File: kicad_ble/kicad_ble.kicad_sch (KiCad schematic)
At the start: 94 parts, among them J2 78171-0002, J3 TC2030_SWD, SW1 RST, SW2 RotaryEncoder_Switch, U1 MAX17048, U2 BQ24075, U3 SRV05-4, U4 nRF52840_E73-2G4M08S1C, U5 74LVC1G11, Y1 32.768 KHz

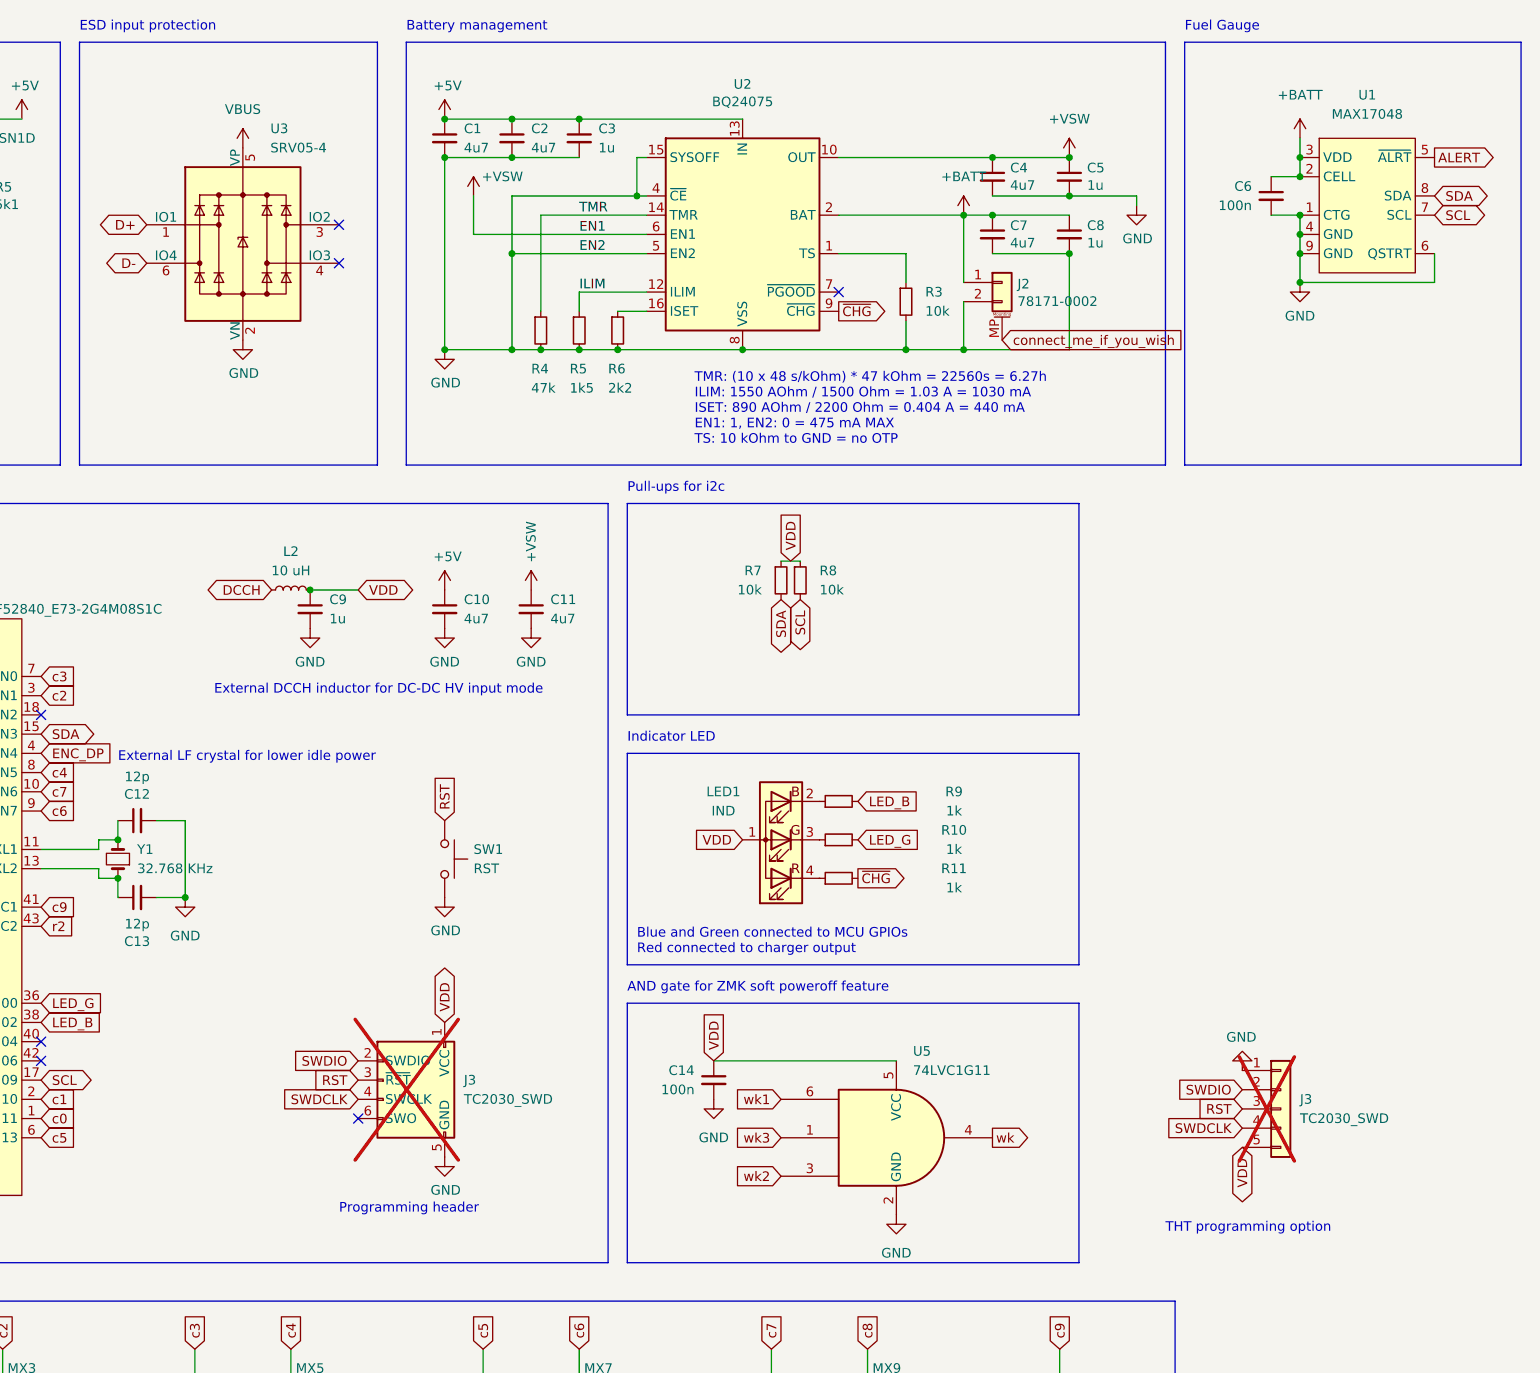
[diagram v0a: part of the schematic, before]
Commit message: next iteration
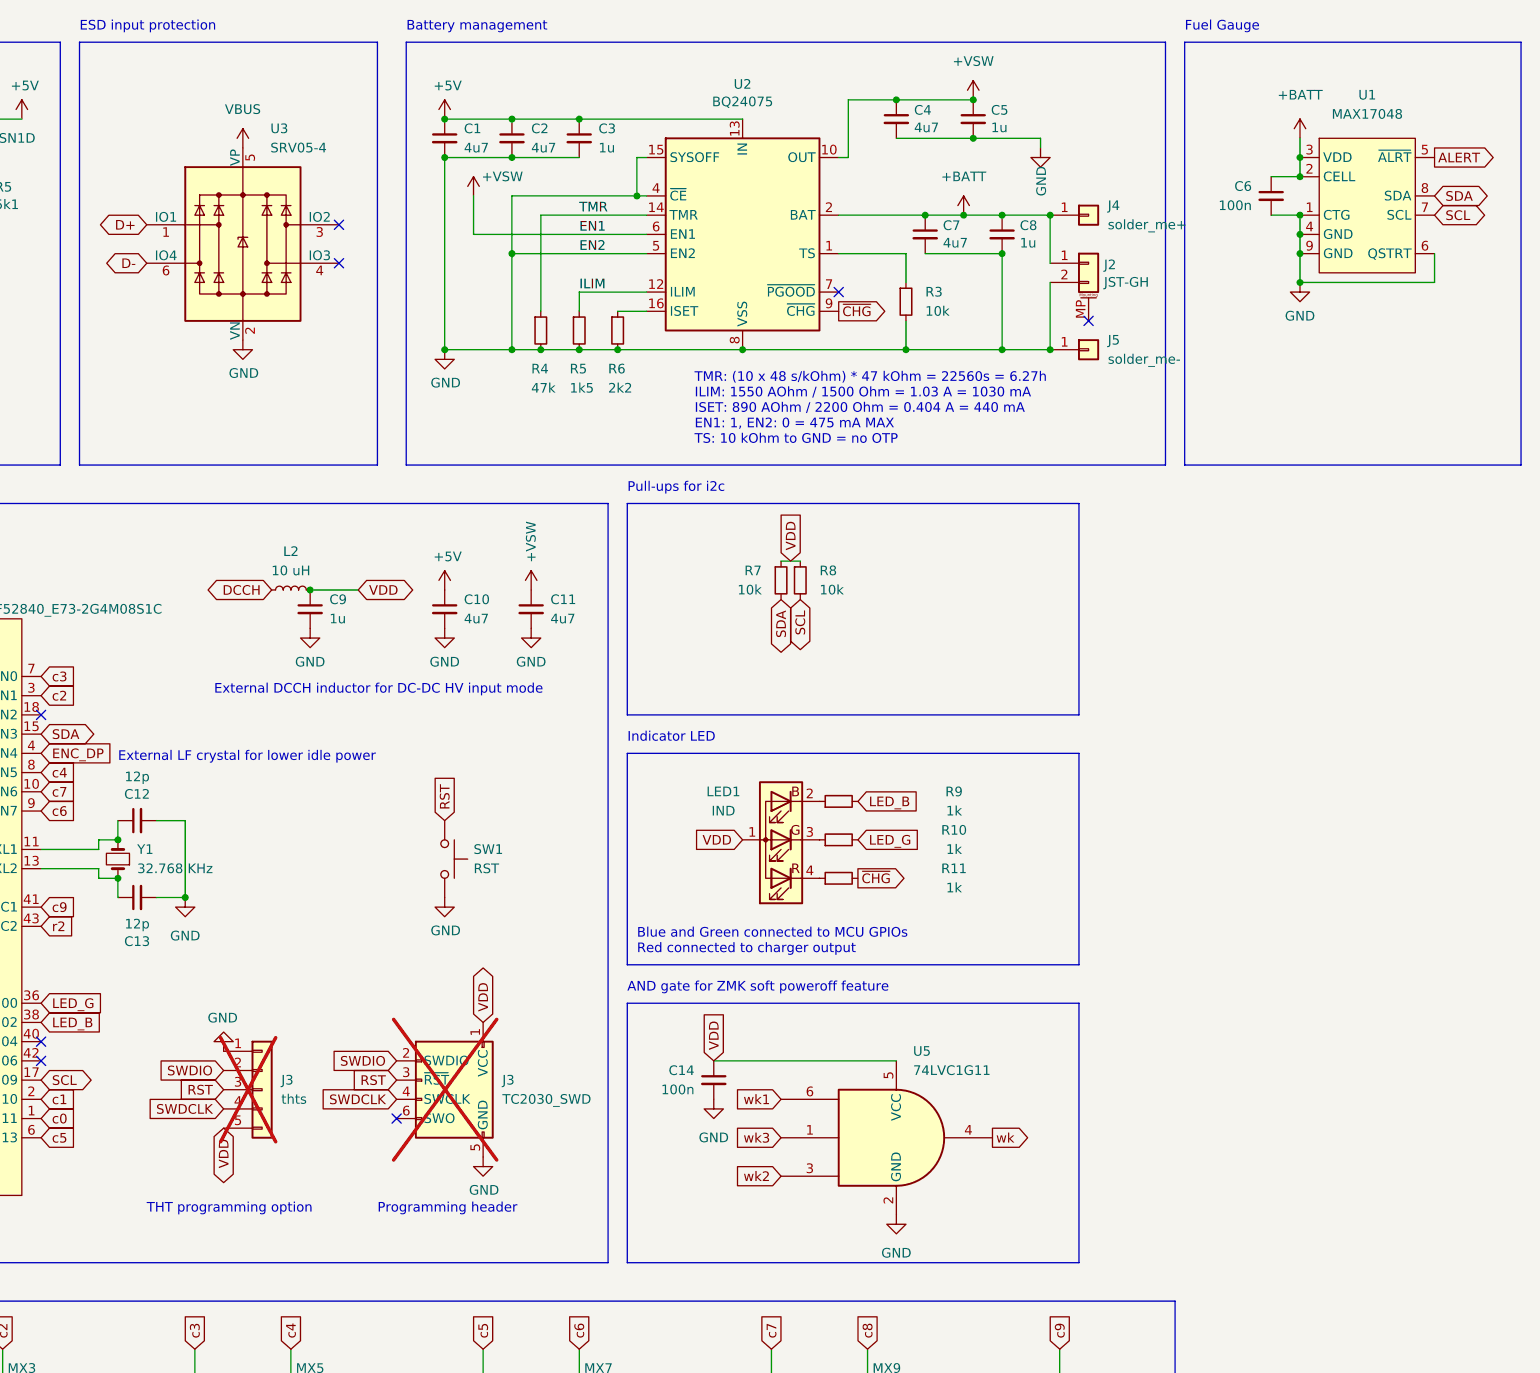
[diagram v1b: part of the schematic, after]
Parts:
- added J4: solder_me+, Connector_Pin:Pin_D0.7mm_L6.5mm_W1.8mm_FlatFork, symbol Connector_Generic:Conn_01x01
- added J5: solder_me-, Connector_PinHeader_2.54mm:PinHeader_1x01_P2.54mm_Vertical, symbol Connector_Generic:Conn_01x01
- J2: value 78171-0002 -> JST-GH; footprint PCM_marbastlib-various:Molex_Pico-EZmate_78171-0002_1x02-1MP_P1.20mm_Vertical -> Connector_JST:JST_GH_SM02B-GHS-TB_1x02-1MP_P1.25mm_Horizontal
- J3: value TC2030_SWD -> thts; now left out of the parts list
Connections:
- net +BATT: now also J4.1 (Pin_1)
- net GND: now also J5.1 (Pin_1)
- net connect_me_if_you_wish: no longer names the net of J2.MP (MountPin)
- no-connect marks 14 -> 15
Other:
- moved on the sheet: C4, C5, C7, C8, J2, J3
